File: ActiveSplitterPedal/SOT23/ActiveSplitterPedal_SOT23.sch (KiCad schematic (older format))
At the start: 9 parts, among them J1 MonoJack2Switch, J2 MonoJack2Switch, J3 MonoJack2Switch, J4 MonoJack2Switch, J5 MonoJack2Switch, J6 Barrel_Jack

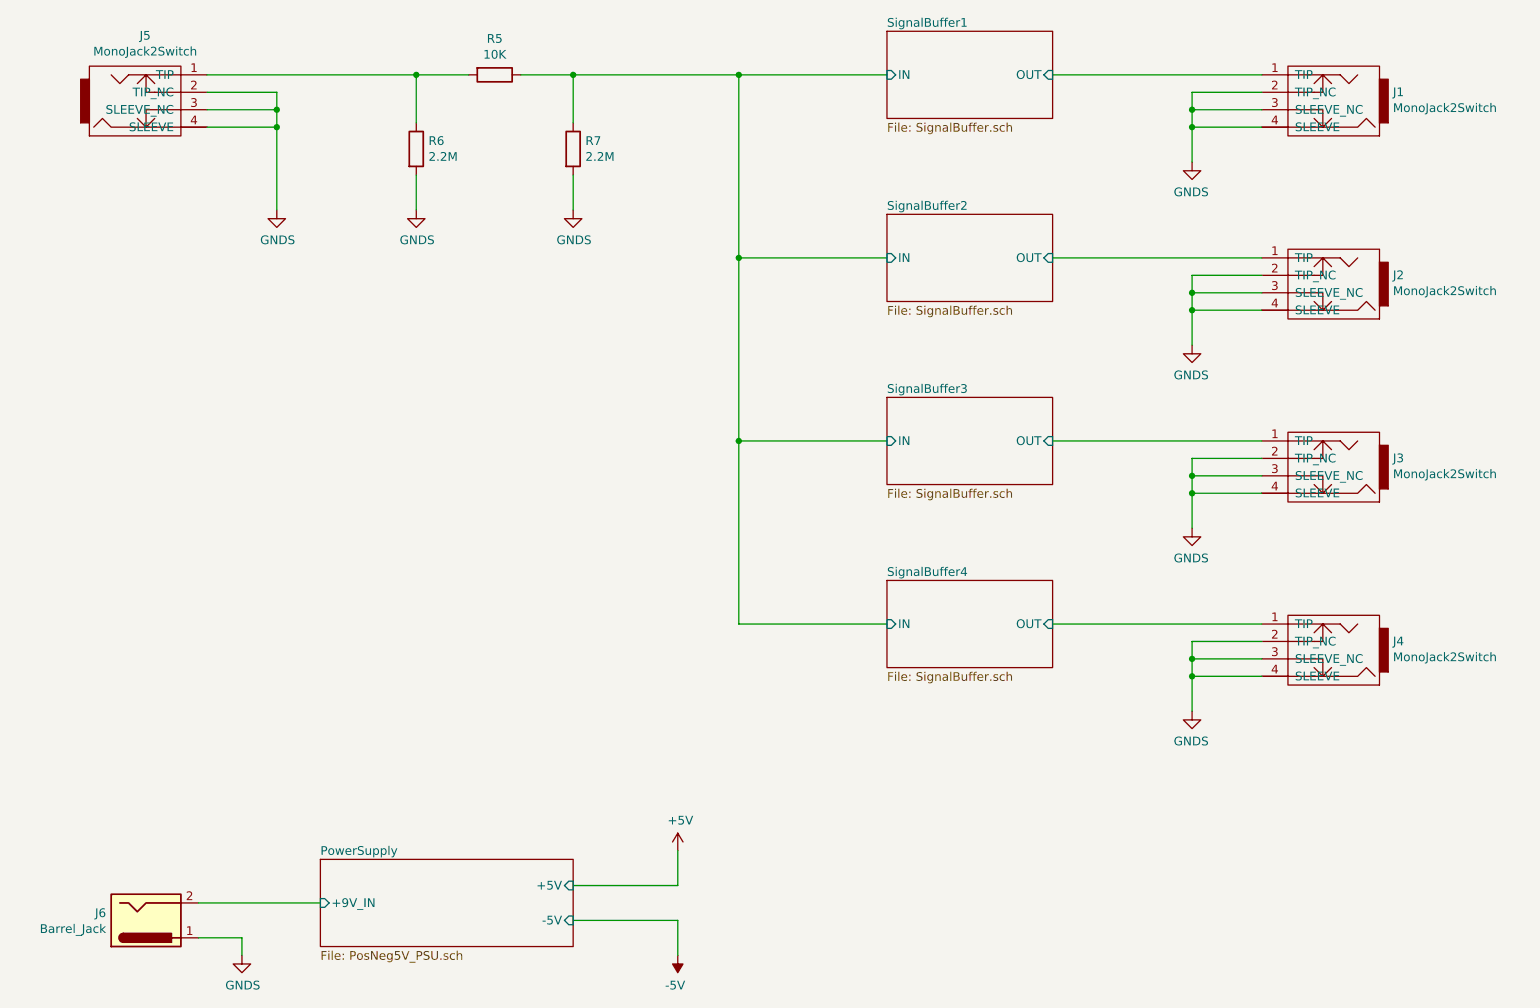
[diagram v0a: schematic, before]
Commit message: Completed RevA layout
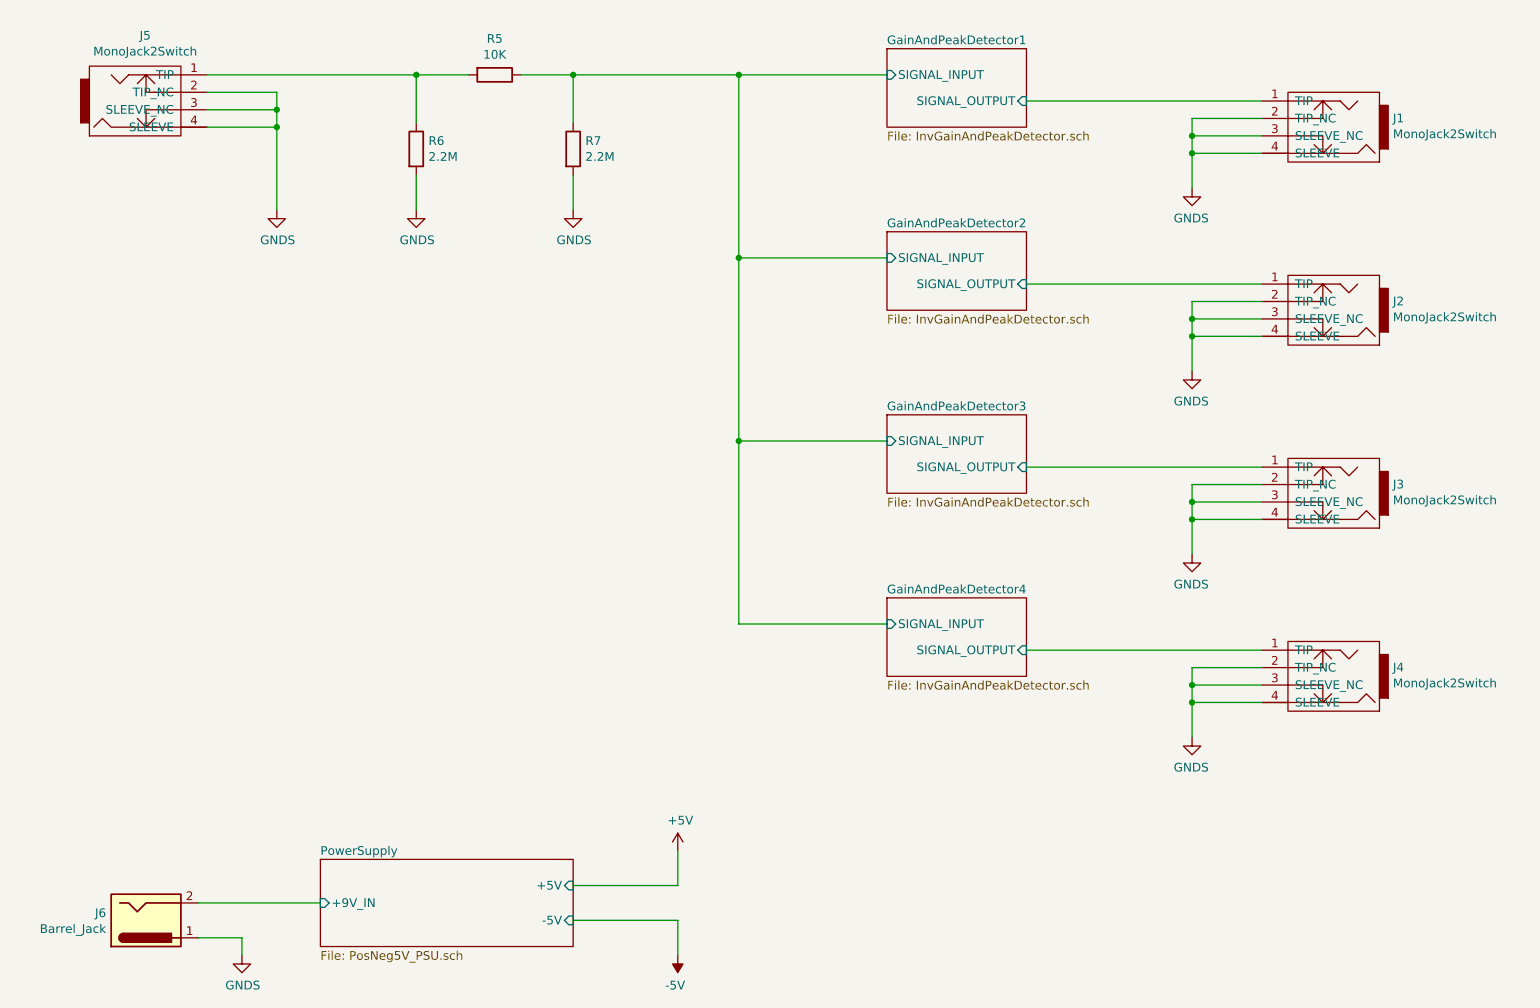
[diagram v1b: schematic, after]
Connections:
- net SignalBuffer1/IN renamed GainAndPeakDetector1/SIGNAL_INPUT
- net SignalBuffer1/OUT renamed GainAndPeakDetector1/SIGNAL_OUTPUT
- net SignalBuffer2/OUT renamed GainAndPeakDetector2/SIGNAL_OUTPUT
- net SignalBuffer3/OUT renamed GainAndPeakDetector3/SIGNAL_OUTPUT
- net SignalBuffer4/OUT renamed GainAndPeakDetector4/SIGNAL_OUTPUT
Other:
- moved on the sheet: J1, J2, J3, J4
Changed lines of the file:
@@
 L MonoJack2Switch:MonoJack2Switch J1
 U 1 1 5F366B64
-P 8950 1450
-F 0 "J1" H 8648 1501 50  0000 R CNN
-F 1 "MonoJack2Switch" H 8648 1410 50  0000 R CNN
-F 2 "NeutrikNRJ:NRJxHx" H 8950 1500 50  0001 C CNN
-F 3 "https://www.neutrik.com/en/product/nrj6hm-1-pre" H 8950 1500 50  0001 C CNN
-	1    8950 1450
+P 8950 1600
+F 0 "J1" H 8648 1651 50  0000 R CNN
+F 1 "MonoJack2Switch" H 8648 1560 50  0000 R CNN
+F 2 "NeutrikNRJ:NRJxHx" H 8950 1650 50  0001 C CNN
+F 3 "https://www.neutrik.com/en/product/nrj6hm-1-pre" H 8950 1650 50  0001 C CNN
+	1    8950 1600
 	-1   0    0    -1
 $EndComp
@@
 L MonoJack2Switch:MonoJack2Switch J2
 U 1 1 5F369E69
-P 8950 2500
-F 0 "J2" H 8648 2551 50  0000 R CNN
-F 1 "MonoJack2Switch" H 8648 2460 50  0000 R CNN
-F 2 "NeutrikNRJ:NRJxHx" H 8950 2550 50  0001 C CNN
-F 3 "https://www.neutrik.com/en/product/nrj6hm-1-pre" H 8950 2550 50  0001 C CNN
-	1    8950 2500
+P 8950 2650
+F 0 "J2" H 8648 2701 50  0000 R CNN
+F 1 "MonoJack2Switch" H 8648 2610 50  0000 R CNN
+F 2 "NeutrikNRJ:NRJxHx" H 8950 2700 50  0001 C CNN
+F 3 "https://www.neutrik.com/en/product/nrj6hm-1-pre" H 8950 2700 50  0001 C CNN
+	1    8950 2650
 	-1   0    0    -1
 $EndComp
@@
 L MonoJack2Switch:MonoJack2Switch J3
 U 1 1 5F36BD50
-P 8950 3550
-F 0 "J3" H 8648 3601 50  0000 R CNN
-F 1 "MonoJack2Switch" H 8648 3510 50  0000 R CNN
-F 2 "NeutrikNRJ:NRJxHx" H 8950 3600 50  0001 C CNN
-F 3 "https://www.neutrik.com/en/product/nrj6hm-1-pre" H 8950 3600 50  0001 C CNN
-	1    8950 3550
+P 8950 3700
+F 0 "J3" H 8648 3751 50  0000 R CNN
+F 1 "MonoJack2Switch" H 8648 3660 50  0000 R CNN
+F 2 "NeutrikNRJ:NRJxHx" H 8950 3750 50  0001 C CNN
+F 3 "https://www.neutrik.com/en/product/nrj6hm-1-pre" H 8950 3750 50  0001 C CNN
+	1    8950 3700
 	-1   0    0    -1
 $EndComp
@@
 L MonoJack2Switch:MonoJack2Switch J4
 U 1 1 5F36CF2A
-P 8950 4600
-F 0 "J4" H 8648 4651 50  0000 R CNN
-F 1 "MonoJack2Switch" H 8648 4560 50  0000 R CNN
-F 2 "NeutrikNRJ:NRJxHx" H 8950 4650 50  0001 C CNN
-F 3 "https://www.neutrik.com/en/product/nrj6hm-1-pre" H 8950 4650 50  0001 C CNN
-	1    8950 4600
+P 8950 4750
+F 0 "J4" H 8648 4801 50  0000 R CNN
+F 1 "MonoJack2Switch" H 8648 4710 50  0000 R CNN
+F 2 "NeutrikNRJ:NRJxHx" H 8950 4800 50  0001 C CNN
+F 3 "https://www.neutrik.com/en/product/nrj6hm-1-pre" H 8950 4800 50  0001 C CNN
+	1    8950 4750
 	-1   0    0    -1
 $EndComp
@@
 $EndComp
 Wire Wire Line
-	8500 1400 8100 1400
-Wire Wire Line
-	8100 1400 8100 1500
-Wire Wire Line
-	8500 1500 8100 1500
-Connection ~ 8100 1500
-Wire Wire Line
-	8100 1500 8100 1600
-Wire Wire Line
-	8500 1600 8100 1600
-Connection ~ 8100 1600
-Wire Wire Line
-	8100 1600 8100 1800
+	8500 1550 8100 1550
+Wire Wire Line
+	8100 1550 8100 1650
+Wire Wire Line
+	8500 1650 8100 1650
+Connection ~ 8100 1650
+Wire Wire Line
+	8100 1650 8100 1750
+Wire Wire Line
+	8500 1750 8100 1750
+Connection ~ 8100 1750
+Wire Wire Line
+	8100 1750 8100 1950
 $Comp
 L power:GNDS #PWR012
 U 1 1 5F3AA43F
-P 8100 1800
-F 0 "#PWR012" H 8100 1550 50  0001 C CNN
-F 1 "GNDS" H 8105 1627 50  0000 C CNN
-F 2 "" H 8100 1800 50  0001 C CNN
-F 3 "" H 8100 1800 50  0001 C CNN
-	1    8100 1800
-	-1   0    0    -1
-$EndComp
-Wire Wire Line
-	8500 2450 8100 2450
-Wire Wire Line
-	8100 2450 8100 2550
-Wire Wire Line
-	8500 2550 8100 2550
-Connection ~ 8100 2550
-Wire Wire Line
-	8100 2550 8100 2650
-Wire Wire Line
-	8500 2650 8100 2650
-Connection ~ 8100 2650
-Wire Wire Line
-	8100 2650 8100 2850
+P 8100 1950
+F 0 "#PWR012" H 8100 1700 50  0001 C CNN
+F 1 "GNDS" H 8105 1777 50  0000 C CNN
+F 2 "" H 8100 1950 50  0001 C CNN
+F 3 "" H 8100 1950 50  0001 C CNN
+	1    8100 1950
+	-1   0    0    -1
+$EndComp
+Wire Wire Line
+	8500 2600 8100 2600
+Wire Wire Line
+	8100 2600 8100 2700
+Wire Wire Line
+	8500 2700 8100 2700
+Connection ~ 8100 2700
+Wire Wire Line
+	8100 2700 8100 2800
+Wire Wire Line
+	8500 2800 8100 2800
+Connection ~ 8100 2800
+Wire Wire Line
+	8100 2800 8100 3000
 $Comp
 L power:GNDS #PWR013
 U 1 1 5F3ABE1D
-P 8100 2850
-F 0 "#PWR013" H 8100 2600 50  0001 C CNN
-F 1 "GNDS" H 8105 2677 50  0000 C CNN
-F 2 "" H 8100 2850 50  0001 C CNN
-F 3 "" H 8100 2850 50  0001 C CNN
-	1    8100 2850
-	-1   0    0    -1
-$EndComp
-Wire Wire Line
-	8500 3500 8100 3500
-Wire Wire Line
-	8100 3500 8100 3600
-Wire Wire Line
-	8500 3600 8100 3600
-Connection ~ 8100 3600
-Wire Wire Line
-	8100 3600 8100 3700
-Wire Wire Line
-	8500 3700 8100 3700
-Connection ~ 8100 3700
-Wire Wire Line
-	8100 3700 8100 3900
+P 8100 3000
+F 0 "#PWR013" H 8100 2750 50  0001 C CNN
+F 1 "GNDS" H 8105 2827 50  0000 C CNN
+F 2 "" H 8100 3000 50  0001 C CNN
+F 3 "" H 8100 3000 50  0001 C CNN
+	1    8100 3000
+	-1   0    0    -1
+$EndComp
+Wire Wire Line
+	8500 3650 8100 3650
+Wire Wire Line
+	8100 3650 8100 3750
+Wire Wire Line
+	8500 3750 8100 3750
+Connection ~ 8100 3750
+Wire Wire Line
+	8100 3750 8100 3850
+Wire Wire Line
+	8500 3850 8100 3850
+Connection ~ 8100 3850
+Wire Wire Line
+	8100 3850 8100 4050
 $Comp
 L power:GNDS #PWR014
 U 1 1 5F3ADB89
-P 8100 3900
-F 0 "#PWR014" H 8100 3650 50  0001 C CNN
-F 1 "GNDS" H 8105 3727 50  0000 C CNN
-F 2 "" H 8100 3900 50  0001 C CNN
-F 3 "" H 8100 3900 50  0001 C CNN
-	1    8100 3900
-	-1   0    0    -1
-$EndComp
-Wire Wire Line
-	8500 4550 8100 4550
-Wire Wire Line
-	8100 4550 8100 4650
-Wire Wire Line
-	8500 4650 8100 4650
-Connection ~ 8100 4650
-Wire Wire Line
-	8100 4650 8100 4750
-Wire Wire Line
-	8500 4750 8100 4750
-Connection ~ 8100 4750
-Wire Wire Line
-	8100 4750 8100 4950
+P 8100 4050
+F 0 "#PWR014" H 8100 3800 50  0001 C CNN
+F 1 "GNDS" H 8105 3877 50  0000 C CNN
+F 2 "" H 8100 4050 50  0001 C CNN
+F 3 "" H 8100 4050 50  0001 C CNN
+	1    8100 4050
+	-1   0    0    -1
+$EndComp
+Wire Wire Line
+	8500 4700 8100 4700
+Wire Wire Line
+	8100 4700 8100 4800
+Wire Wire Line
+	8500 4800 8100 4800
+Connection ~ 8100 4800
+Wire Wire Line
+	8100 4800 8100 4900
+Wire Wire Line
+	8500 4900 8100 4900
+Connection ~ 8100 4900
+Wire Wire Line
+	8100 4900 8100 5100
 $Comp
 L power:GNDS #PWR015
 U 1 1 5F3AF94C
-P 8100 4950
-F 0 "#PWR015" H 8100 4700 50  0001 C CNN
-F 1 "GNDS" H 8105 4777 50  0000 C CNN
-F 2 "" H 8100 4950 50  0001 C CNN
-F 3 "" H 8100 4950 50  0001 C CNN
-	1    8100 4950
+P 8100 5100
+F 0 "#PWR015" H 8100 4850 50  0001 C CNN
+F 1 "GNDS" H 8105 4927 50  0000 C CNN
+F 2 "" H 8100 5100 50  0001 C CNN
+F 3 "" H 8100 5100 50  0001 C CNN
+	1    8100 5100
 	-1   0    0    -1
 $EndComp
@@
 $EndSheet
 Wire Wire Line
-	7300 2350 8500 2350
-Wire Wire Line
-	7300 3400 8500 3400
-Wire Wire Line
-	7300 4450 8500 4450
-Wire Wire Line
-	7300 1300 8500 1300
+	7150 2500 8500 2500
+Wire Wire Line
+	7150 3550 8500 3550
+Wire Wire Line
+	7150 4600 8500 4600
+Wire Wire Line
+	7150 1450 8500 1450
 Wire Wire Line
 	4550 1300 5500 1300
@@
 	5500 4450 6350 4450
 $Sheet
-S 6350 4200 950  500
-U 5F365B82
-F0 "SignalBuffer4" 50
-F1 "SignalBuffer.sch" 50
-F2 "IN" I L 6350 4450 50
-F3 "OUT" I R 7300 4450 50
-$EndSheet
-$Sheet
-S 6350 3150 950  500
-U 5F365961
-F0 "SignalBuffer3" 50
-F1 "SignalBuffer.sch" 50
-F2 "IN" I L 6350 3400 50
-F3 "OUT" I R 7300 3400 50
-$EndSheet
-$Sheet
-S 6350 2100 950  500
-U 5F3658F9
-F0 "SignalBuffer2" 50
-F1 "SignalBuffer.sch" 50
-F2 "IN" I L 6350 2350 50
-F3 "OUT" I R 7300 2350 50
-$EndSheet
-$Sheet
-S 6350 1050 950  500
-U 5F350192
-F0 "SignalBuffer1" 50
-F1 "SignalBuffer.sch" 50
-F2 "IN" I L 6350 1300 50
-F3 "OUT" I R 7300 1300 50
+S 6350 2200 800  450
+U 5F512144
+F0 "GainAndPeakDetector2" 50
+F1 "InvGainAndPeakDetector.sch" 50
+F2 "SIGNAL_INPUT" I L 6350 2350 50
+F3 "SIGNAL_OUTPUT" I R 7150 2500 50
+$EndSheet
+$Sheet
+S 6350 3250 800  450
+U 5F515E89
+F0 "GainAndPeakDetector3" 50
+F1 "InvGainAndPeakDetector.sch" 50
+F2 "SIGNAL_INPUT" I L 6350 3400 50
+F3 "SIGNAL_OUTPUT" I R 7150 3550 50
+$EndSheet
+$Sheet
+S 6350 4300 800  450
+U 5F519B24
+F0 "GainAndPeakDetector4" 50
+F1 "InvGainAndPeakDetector.sch" 50
+F2 "SIGNAL_INPUT" I L 6350 4450 50
+F3 "SIGNAL_OUTPUT" I R 7150 4600 50
+$EndSheet
+$Sheet
+S 6350 1150 800  450
+U 5F3F1F31
+F0 "GainAndPeakDetector1" 50
+F1 "InvGainAndPeakDetector.sch" 50
+F2 "SIGNAL_INPUT" I L 6350 1300 50
+F3 "SIGNAL_OUTPUT" I R 7150 1450 50
 $EndSheet
 $EndSCHEMATC
